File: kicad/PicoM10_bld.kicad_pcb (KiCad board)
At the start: 6 copper layers, 8 x 10 mm, 20 parts, among them J1 Conn_Coaxial, U1 MIA-M10Q, U2 NCP160xMX

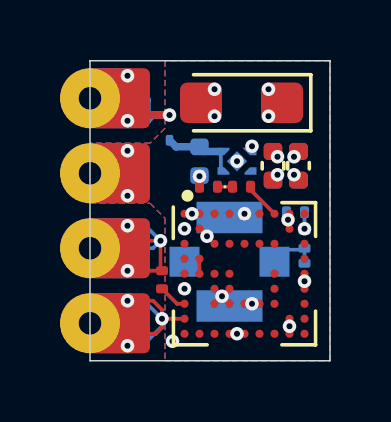
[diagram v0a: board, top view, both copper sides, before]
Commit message: minor schematic and layout updates
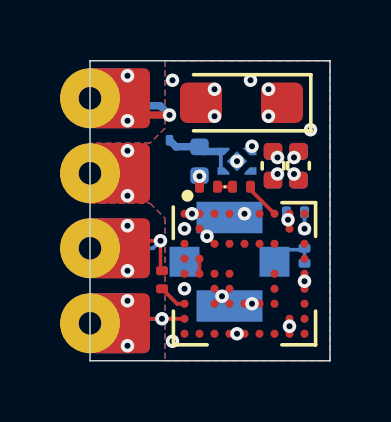
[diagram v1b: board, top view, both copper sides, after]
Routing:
- net GNSS_Rx: track 7.94 -> 4.77 mm
- net Net-(R1-Pad1): track 6.63 -> 4.18 mm
- net Net-(D1-A): track 4.77 -> 3.81 mm
- net GND: vias 18 -> 21
